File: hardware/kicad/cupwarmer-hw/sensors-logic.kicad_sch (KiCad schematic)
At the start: 3 parts, among them J1 I2C Service

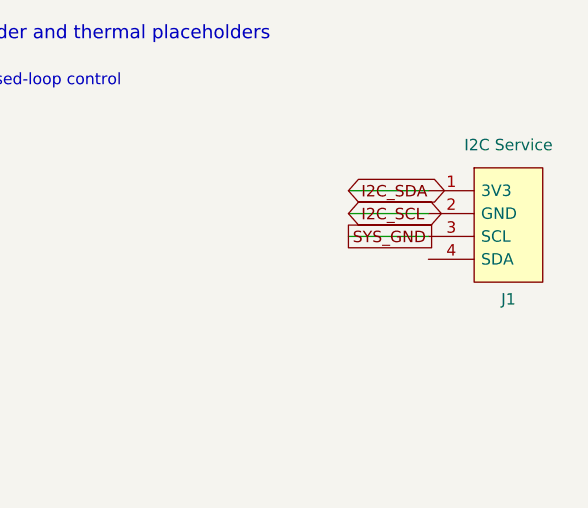
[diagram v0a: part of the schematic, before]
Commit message: Update hardware schematics and BOM
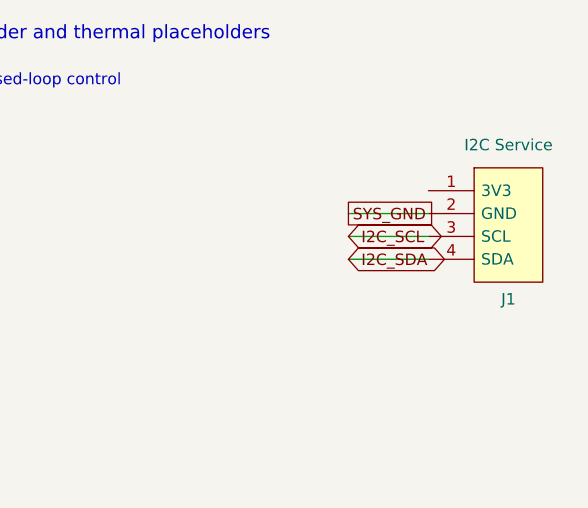
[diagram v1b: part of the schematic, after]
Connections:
- net I2C_SCL: now also J1.3 (SCL); no longer J1.2 (GND)
- net I2C_SDA: now also J1.4 (SDA); no longer J1.1 (3V3)
- net SYS_GND: now also J1.2 (GND); no longer J1.3 (SCL)
